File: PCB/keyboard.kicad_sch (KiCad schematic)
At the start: 153 parts, among them J1 JST SH 4-pin, SW1 SW_Push, U1 ATmega32U4-A, U2 SRV05-4, Y1 16MHz

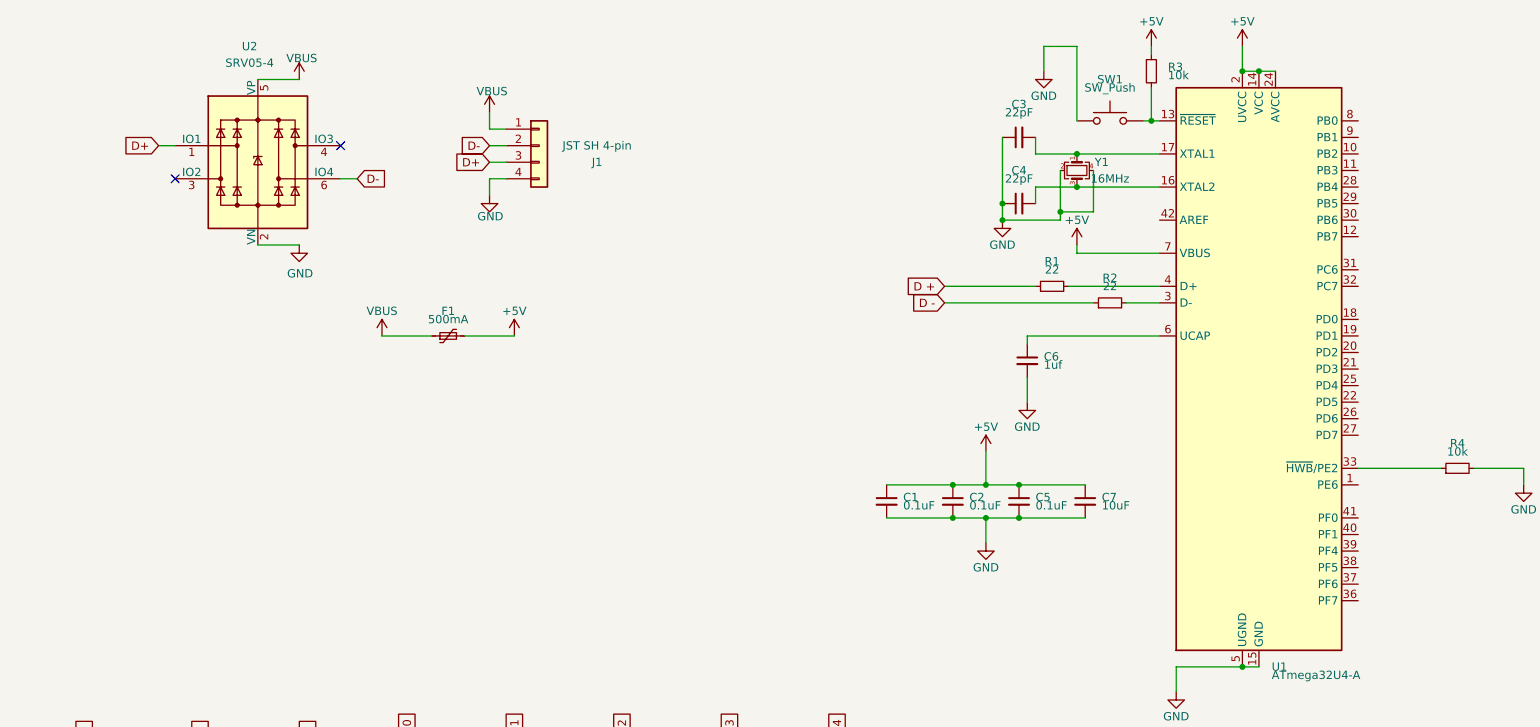
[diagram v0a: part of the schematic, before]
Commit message: Working on traces
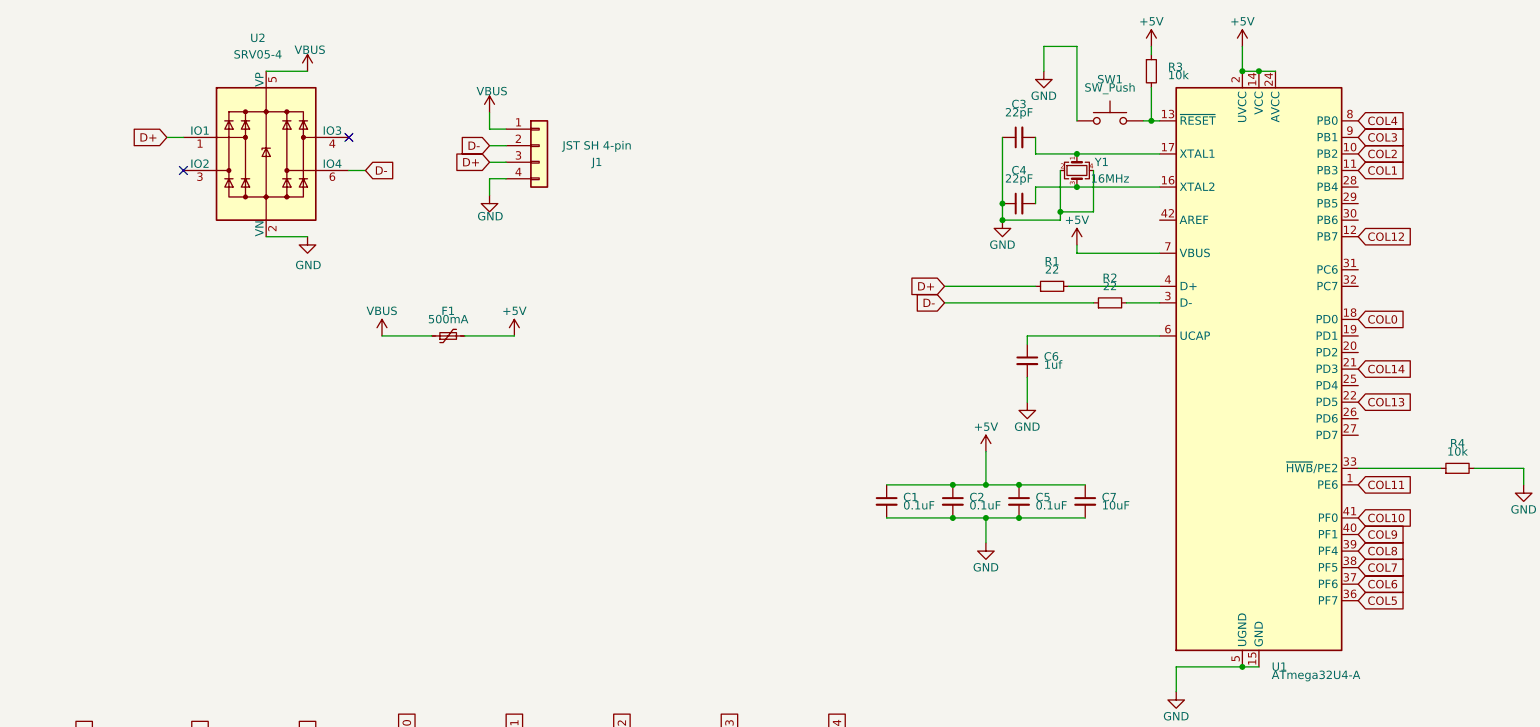
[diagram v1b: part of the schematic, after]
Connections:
- net D + is gone; now on net D+: R1.1
- net D - is gone; now on net D-: R2.1
- net COL0: now also U1.18 (PD0)
- net COL1: now also U1.11 (PB3)
- net COL10: now also U1.41 (PF0)
- net COL11: now also U1.1 (PE6)
- net COL12: now also U1.12 (PB7)
- net COL13: now also U1.22 (PD5)
- net COL14: now also U1.21 (PD3)
- net COL2: now also U1.10 (PB2)
- net COL3: now also U1.9 (PB1)
- net COL4: now also U1.8 (PB0)
- net COL5: now also U1.36 (PF7)
- net COL6: now also U1.37 (PF6)
- net COL7: now also U1.38 (PF5)
- net COL8: now also U1.39 (PF4)
- net COL9: now also U1.40 (PF1)
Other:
- moved on the sheet: U2

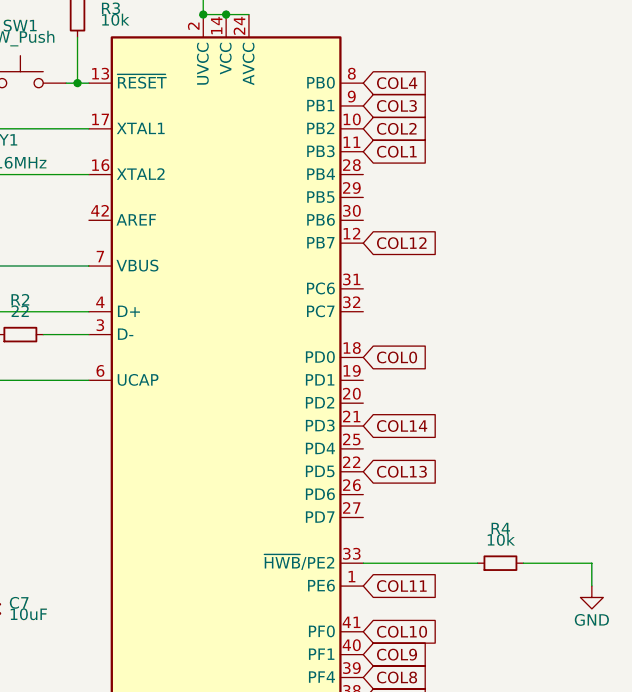
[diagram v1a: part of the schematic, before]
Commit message: finnished traces
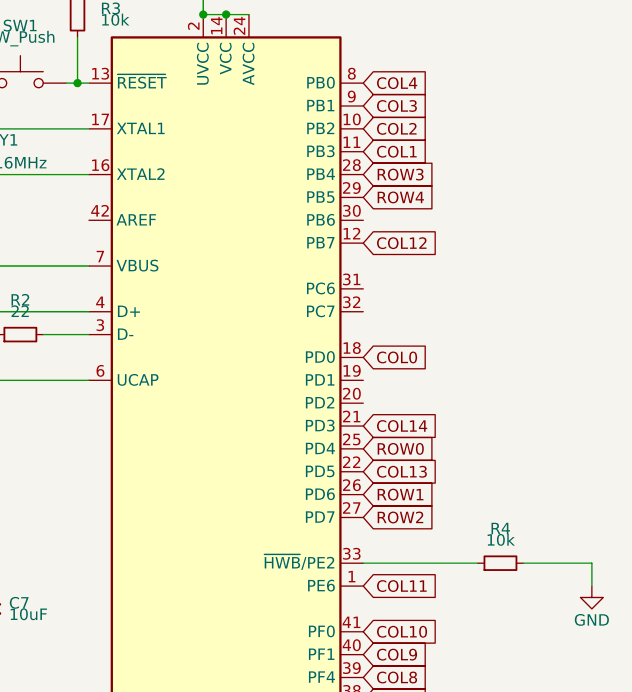
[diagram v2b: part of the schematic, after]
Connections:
- net ROW0: now also U1.25 (PD4)
- net ROW1: now also U1.26 (PD6)
- net ROW2: now also U1.27 (PD7)
- net ROW3: now also U1.28 (PB4)
- net ROW4: now also U1.29 (PB5)
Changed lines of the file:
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@@
+    )
+  )
+  (global_label "ROW1" (shape input) (at 373.38 80.01 0) (fields_autoplaced)
+    (effects (font (size 1.27 1.27)) (justify left))
+    (property "Intersheetrefs" "${INTERSHEET_REFS}" (id 0) (at 380.988 80.01 0)
+      (effects (font (size 1.27 1.27)) (justify left) hide)
     )
   )
@@
     (effects (font (size 1.27 1.27)) (justify left))
     (property "Intersheetrefs" "${INTERSHEET_REFS}" (id 0) (at 106.68 126.1653 90)
+      (effects (font (size 1.27 1.27)) (justify left) hide)
+    )
+  )
+  (global_label "ROW0" (shape input) (at 373.38 74.93 0) (fields_autoplaced)
+    (effects (font (size 1.27 1.27)) (justify left))
+    (property "Intersheetrefs" "${INTERSHEET_REFS}" (id 0) (at 380.988 74.93 0)
       (effects (font (size 1.27 1.27)) (justify left) hide)
     )
@@
     )
   )
+  (global_label "ROW2" (shape input) (at 373.38 82.55 0) (fields_autoplaced)
+    (effects (font (size 1.27 1.27)) (justify left))
+    (property "Intersheetrefs" "${INTERSHEET_REFS}" (id 0) (at 380.988 82.55 0)
+      (effects (font (size 1.27 1.27)) (justify left) hide)
+    )
+  )
   (global_label "COL7" (shape input) (at 373.38 102.87 0) (fields_autoplaced)
     (effects (font (size 1.27 1.27)) (justify left))
@@
     )
   )
+  (global_label "ROW4" (shape input) (at 373.38 46.99 0) (fields_autoplaced)
+    (effects (font (size 1.27 1.27)) (justify left))
+    (property "Intersheetrefs" "${INTERSHEET_REFS}" (id 0) (at 380.988 46.99 0)
+      (effects (font (size 1.27 1.27)) (justify left) hide)
+    )
+  )
   (global_label "COL10" (shape input) (at 373.38 95.25 0) (fields_autoplaced)
     (effects (font (size 1.27 1.27)) (justify left))
@@
       (effects (font (size 1.27 1.27)) (justify left) hide)
     )
+  )
+  (global_label "ROW3" (shape input) (at 373.38 44.45 0) (fields_autoplaced)
+    (effects (font (size 1.27 1.27)) (justify left))
+    (property "Intersheetrefs" "${INTERSHEET_REFS}" (id 0) (at 380.988 44.45 0)
+      (effects (font (size 1.27 1.27)) (justify left) hide)
+    )
